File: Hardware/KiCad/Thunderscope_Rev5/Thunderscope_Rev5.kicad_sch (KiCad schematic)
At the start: 10 parts

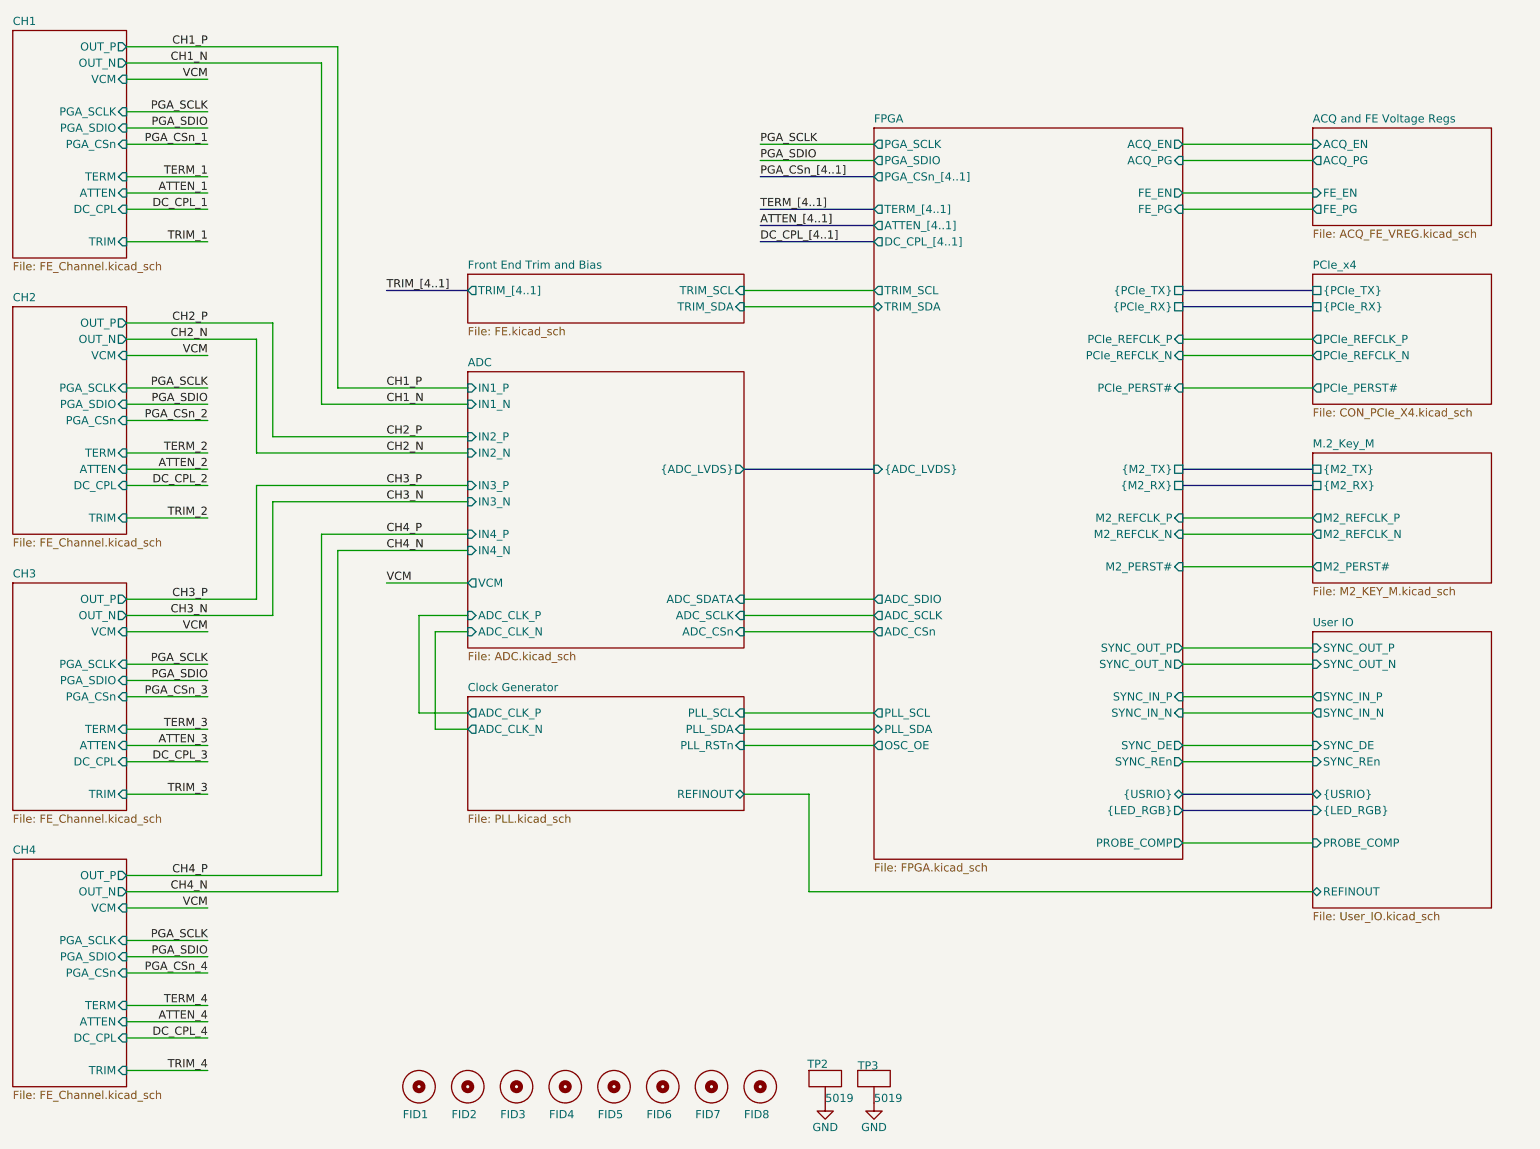
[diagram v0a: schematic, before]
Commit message: Refactored Schematic
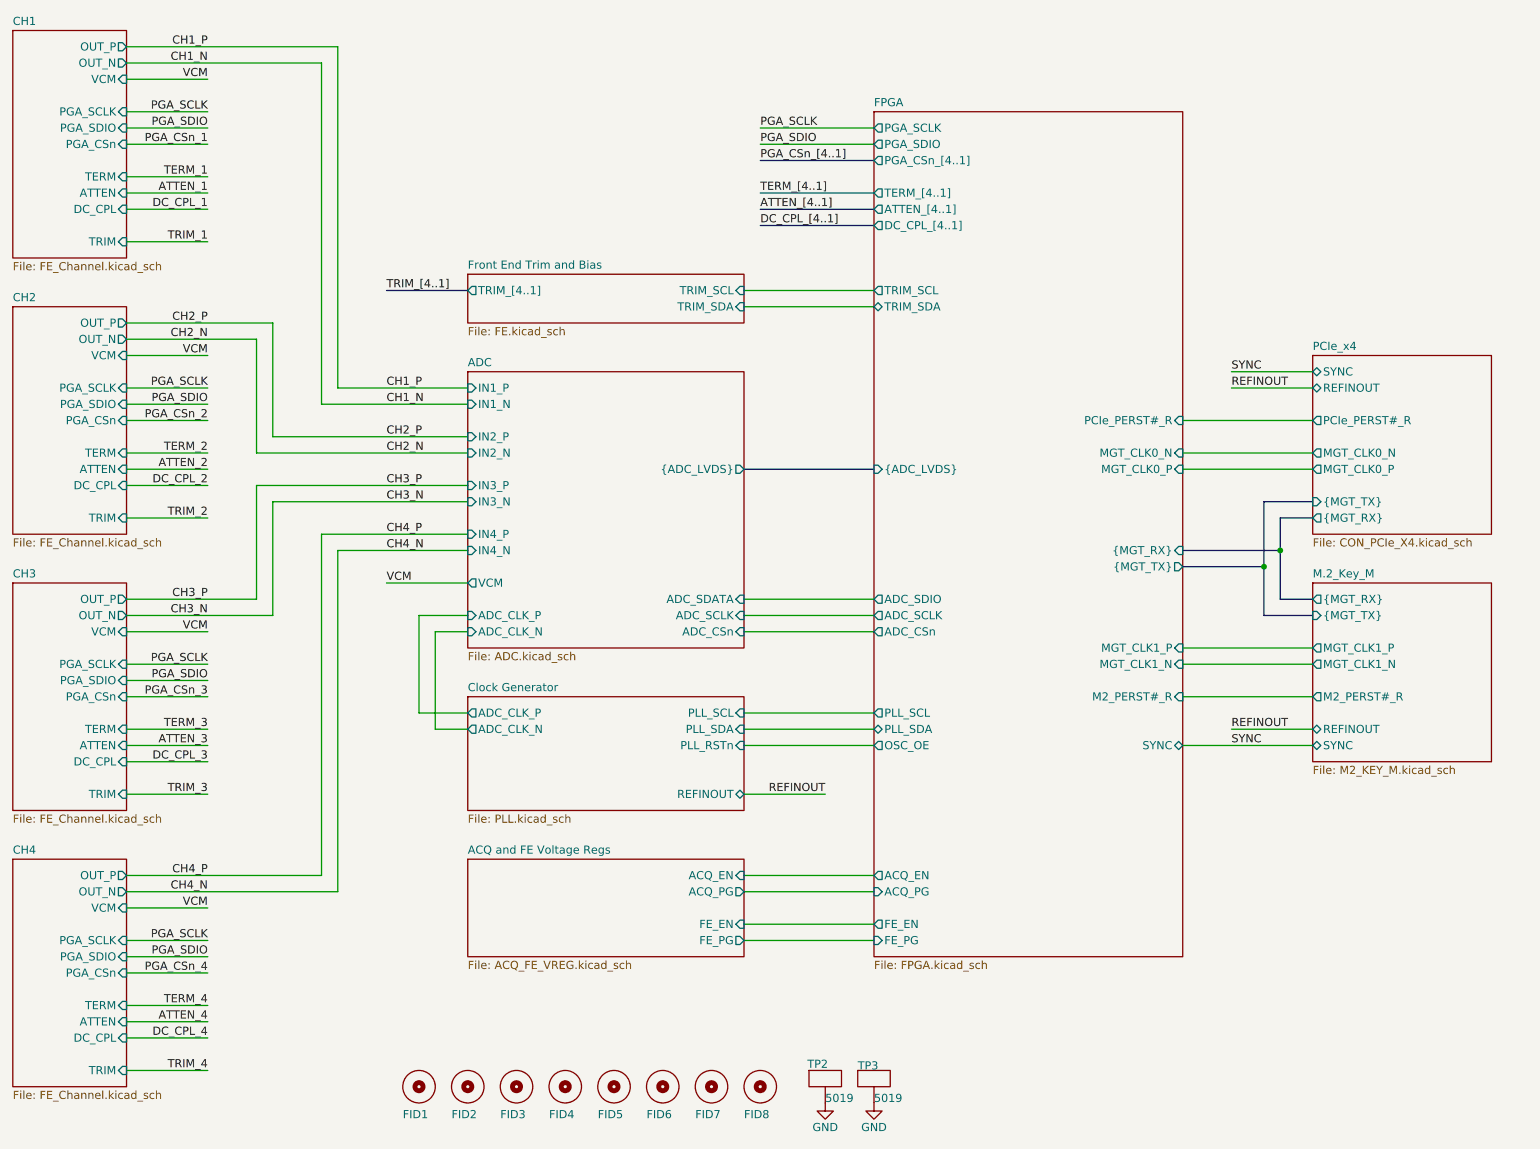
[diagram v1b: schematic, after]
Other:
- removed sheet User IO
- sheet FPGA ports: added M2_PERST#_R, MGT_CLK0_N, MGT_CLK0_P, MGT_CLK1_N, MGT_CLK1_P, PCIe_PERST#_R, SYNC, {MGT_RX}, {MGT_TX}; removed M2_PERST#, M2_REFCLK_N, M2_REFCLK_P, PCIe_PERST#, PCIe_REFCLK_N, PCIe_REFCLK_P, PROBE_COMP, SYNC_DE, SYNC_IN_N, SYNC_IN_P, SYNC_OUT_N, SYNC_OUT_P, SYNC_REn, {LED_RGB}, {M2_RX}, {M2_TX}, {PCIe_RX}, {PCIe_TX}, {USRIO}
- sheet M.2_Key_M ports: added M2_PERST#_R, MGT_CLK1_N, MGT_CLK1_P, REFINOUT, SYNC, {MGT_RX}, {MGT_TX}; removed M2_PERST#, M2_REFCLK_N, M2_REFCLK_P, {M2_RX}, {M2_TX}
- sheet PCIe_x4 ports: added MGT_CLK0_N, MGT_CLK0_P, PCIe_PERST#_R, REFINOUT, SYNC, {MGT_RX}, {MGT_TX}; removed PCIe_PERST#, PCIe_REFCLK_N, PCIe_REFCLK_P, {PCIe_RX}, {PCIe_TX}
